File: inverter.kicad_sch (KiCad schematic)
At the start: 28 parts, among them Q1 IRF530NPBF, Q2 IRF530NPBF, Q3 IRF530NPBF, Q4 IRF530NPBF, U1 IR2110, U2 IR2110

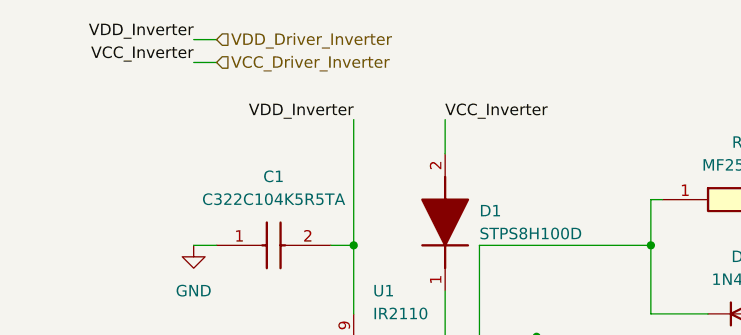
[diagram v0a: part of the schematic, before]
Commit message: SCH Save: 2 files changed GateDriver.kicad_sch 0/0/2 inverter.kicad_sch 0/0/2
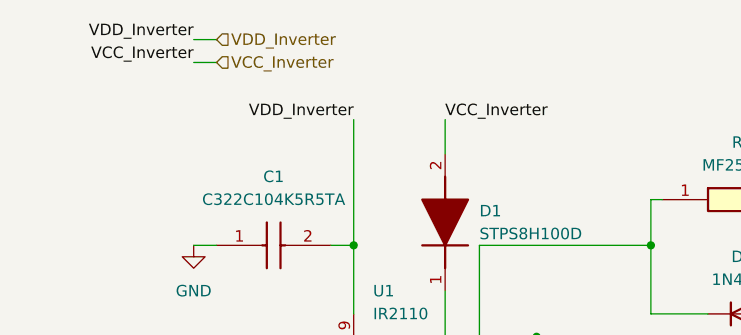
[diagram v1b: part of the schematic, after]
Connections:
- net VCC_Driver_Inverter renamed VCC_Inverter
- net VDD_Driver_Inverter renamed VDD_Inverter
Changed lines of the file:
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@@
 		)
 	)
-	(hierarchical_label "VDD_Driver_Inverter"
+	(hierarchical_label "VDD_Inverter"
 		(shape input)
 		(at 29.21 16.51 0)
@@
 		)
 	)
-	(hierarchical_label "VCC_Driver_Inverter"
+	(hierarchical_label "VCC_Inverter"
 		(shape input)
 		(at 29.21 19.05 0)

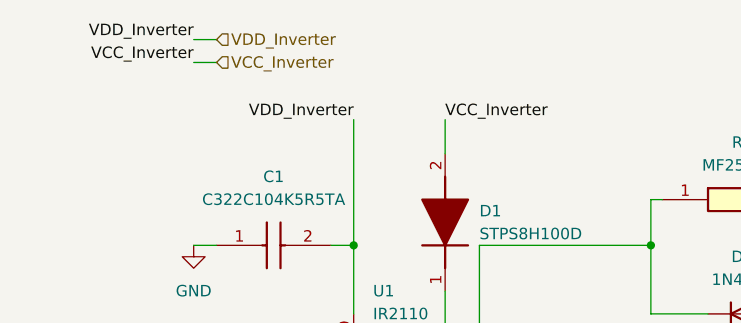
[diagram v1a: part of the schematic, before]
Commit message: Autosave
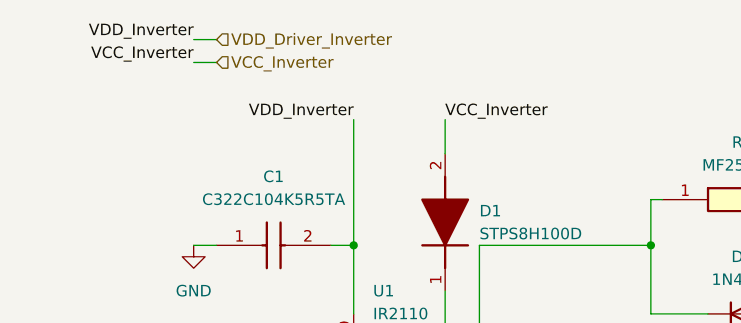
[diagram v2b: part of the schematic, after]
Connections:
- net VDD_Inverter renamed VDD_Driver_Inverter
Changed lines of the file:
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@@
 		)
 	)
-	(hierarchical_label "VDD_Inverter"
+	(hierarchical_label "VDD_Driver_Inverter"
 		(shape input)
 		(at 29.21 16.51 0)

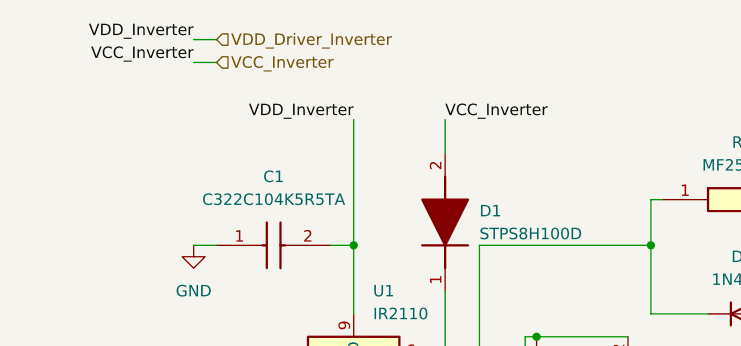
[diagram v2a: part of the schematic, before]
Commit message: Autosave
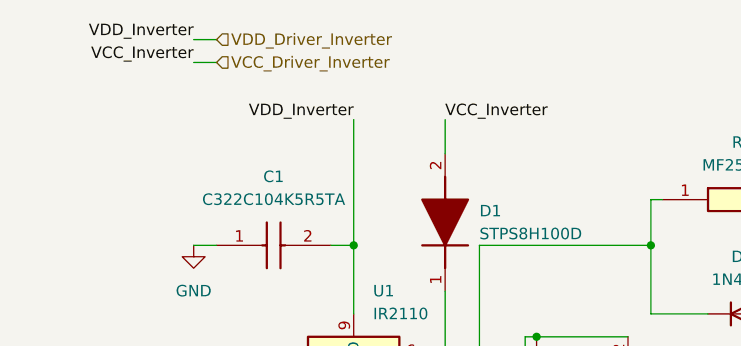
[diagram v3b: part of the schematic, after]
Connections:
- net VCC_Inverter renamed VCC_Driver_Inverter
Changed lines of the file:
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@@
 		)
 	)
-	(hierarchical_label "VCC_Inverter"
+	(hierarchical_label "VCC_Driver_Inverter"
 		(shape input)
 		(at 29.21 19.05 0)

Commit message: SCH Save: 1 files changed inverter.kicad_sch 0/0/15
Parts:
- C3: footprint (none) -> Capacitor_THT:C_Rect_L7.0mm_W2.5mm_P5.00mm
- D1, D4: footprint (none) -> Package_TO_SOT_THT:TO-220-2_Vertical
- Q1, Q2, Q3, Q4: footprint (none) -> Package_TO_SOT_THT:TO-220-3_Vertical
- R10, R11, R12, R13, R14, R15, R16, R9: footprint (none) -> Resistor_THT:R_Axial_DIN0207_L6.3mm_D2.5mm_P7.62mm_Horizontal
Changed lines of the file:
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@@
 			)
 		)
-		(property "Footprint" ""
+		(property "Footprint" "Package_TO_SOT_THT:TO-220-3_Vertical"
 			(at 132.08 166.04 0)
 			(hide yes)
@@
 			)
 		)
-		(property "Footprint" ""
+		(property "Footprint" "Resistor_THT:R_Axial_DIN0207_L6.3mm_D2.5mm_P7.62mm_Horizontal"
 			(at 201.93 160.96 0)
 			(hide yes)
@@
 			)
 		)
-		(property "Footprint" ""
+		(property "Footprint" "Package_TO_SOT_THT:TO-220-3_Vertical"
 			(at 162.56 166.04 0)
 			(hide yes)
@@
 			)
 		)
-		(property "Footprint" ""
+		(property "Footprint" "Resistor_THT:R_Axial_DIN0207_L6.3mm_D2.5mm_P7.62mm_Horizontal"
 			(at 91.77 68.58 0)
 			(hide yes)
@@
 			)
 		)
-		(property "Footprint" ""
+		(property "Footprint" "Package_TO_SOT_THT:TO-220-3_Vertical"
 			(at 132.08 134.29 0)
 			(hide yes)
@@
 			)
 		)
-		(property "Footprint" ""
+		(property "Footprint" "Resistor_THT:R_Axial_DIN0207_L6.3mm_D2.5mm_P7.62mm_Horizontal"
 			(at 202.87 39.37 0)
 			(hide yes)
@@
 			)
 		)
-		(property "Footprint" ""
+		(property "Footprint" "Resistor_THT:R_Axial_DIN0207_L6.3mm_D2.5mm_P7.62mm_Horizontal"
 			(at 92.71 160.96 0)
 			(hide yes)
@@
 			)
 		)
-		(property "Footprint" ""
+		(property "Footprint" "Resistor_THT:R_Axial_DIN0207_L6.3mm_D2.5mm_P7.62mm_Horizontal"
 			(at 202.87 68.58 0)
 			(hide yes)
@@
 			)
 		)
-		(property "Footprint" ""
+		(property "Footprint" "Package_TO_SOT_THT:TO-220-2_Vertical"
 			(at 142.57 33.02 0)
 			(hide yes)
@@
 			)
 		)
-		(property "Footprint" ""
+		(property "Footprint" "Capacitor_THT:C_Rect_L7.0mm_W2.5mm_P5.00mm"
 			(at 149.86 149.53 0)
 			(hide yes)
@@
 			)
 		)
-		(property "Footprint" ""
+		(property "Footprint" "Resistor_THT:R_Axial_DIN0207_L6.3mm_D2.5mm_P7.62mm_Horizontal"
 			(at 92.71 130.48 0)
 			(hide yes)
@@
 			)
 		)
-		(property "Footprint" ""
+		(property "Footprint" "Resistor_THT:R_Axial_DIN0207_L6.3mm_D2.5mm_P7.62mm_Horizontal"
 			(at 91.77 39.37 0)
 			(hide yes)
@@
 			)
 		)
-		(property "Footprint" ""
+		(property "Footprint" "Resistor_THT:R_Axial_DIN0207_L6.3mm_D2.5mm_P7.62mm_Horizontal"
 			(at 201.93 130.48 0)
 			(hide yes)
@@
 			)
 		)
-		(property "Footprint" ""
+		(property "Footprint" "Package_TO_SOT_THT:TO-220-2_Vertical"
 			(at 152.07 33.02 0)
 			(hide yes)
@@
 			)
 		)
-		(property "Footprint" ""
+		(property "Footprint" "Package_TO_SOT_THT:TO-220-3_Vertical"
 			(at 162.56 134.29 0)
 			(hide yes)
